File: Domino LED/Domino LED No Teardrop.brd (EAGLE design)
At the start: 27.9 x 10.2 mm, 23 parts, among them J1 MH11-1

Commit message: Changed copyright
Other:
- board text added: "Reference designs are provided "AS IS" and "WITH ALL FAULTS". The Domino Team disclaims all other warranties express or implied, regarding this product, including but not limited to, any implied warranties of merchantibility or fitness for any particular application."
- board text added: "The Domino Team may make changes to specifications and product descriptions at any time, without notice."
- board text added: "© 2014, The Domino Team. All rights reserved."
- board text removed: "Michel Stempin may make changes to specifications and product descriptions at any time, without notice."
- board text removed: "Reference designs are provided "AS IS" and "WITH ALL FAULTS". Michel Stempin disclaims all other warranties express or implied, regarding this product, including but not limited to, any implied warranties of merchantibility or fitness for any particular application."
- board text removed: "© 2014, Michel Stempin. All rights reserved."
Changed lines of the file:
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@@
 See creativecommons.org/licenses/by-sa/4.0/</text>
 <text x="34.29" y="-51.943" size="0.8128" layer="48" ratio="20">Reference designs are provided "AS IS" and "WITH ALL FAULTS".
-Michel Stempin disclaims all other warranties express or implied,
+The Domino Team disclaims all other warranties express or implied,
 regarding this product, including but not limited to, any implied warranties of
 merchantibility or fitness for any particular application.</text>
-<text x="34.29" y="-55.753" size="0.8128" layer="48" ratio="20">Michel Stempin may make changes to specifications and product descriptions
+<text x="34.29" y="-55.753" size="0.8128" layer="48" ratio="20">The Domino Team may make changes to specifications and product descriptions
 at any time, without notice.</text>
-<text x="74.93" y="-41.91" size="1.27" layer="48" ratio="20">© 2014, Michel Stempin.
+<text x="74.93" y="-41.91" size="1.27" layer="48" ratio="20">© 2014, The Domino Team.
 All rights reserved.</text>
 <text x="115.57" y="-57.15" size="1.778" layer="48">Rev.</text>

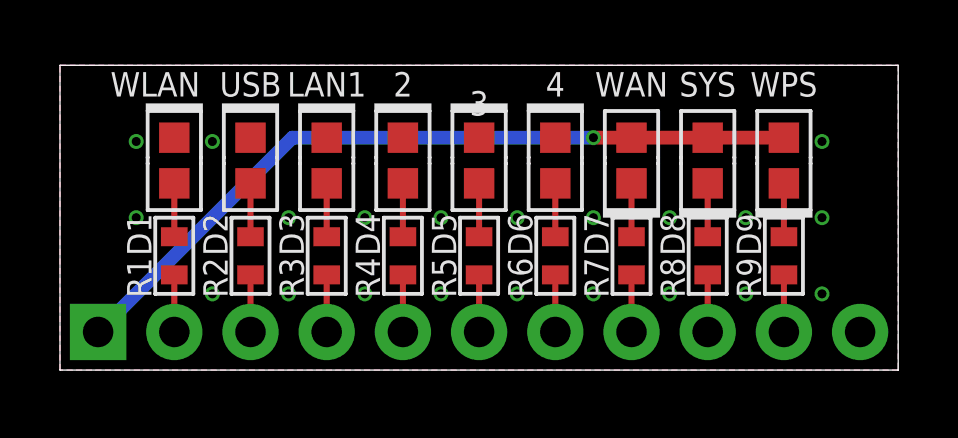
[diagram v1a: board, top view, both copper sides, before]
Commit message: ... and all the files I missed
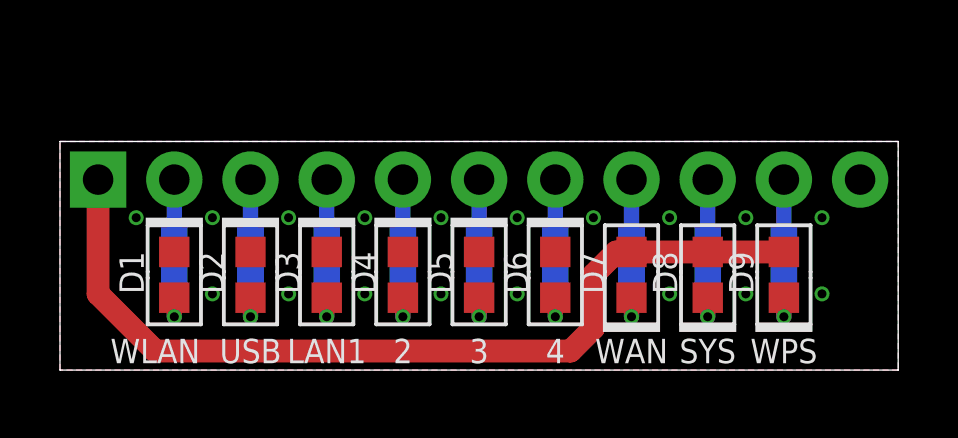
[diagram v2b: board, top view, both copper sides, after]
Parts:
- removed U$4: (no value), Domino:DOMINO_LOGO_SMALL
- moved J1 5.08 mm to (1.27, 6.35)
- moved D1 3.81 mm to (3.81, 3.17)
- moved D2 3.81 mm to (6.35, 3.17)
- moved D3 3.81 mm to (8.89, 3.17)
- moved D4 3.81 mm to (11.4, 3.17)
- moved D5 3.81 mm to (14.0, 3.17)
- moved D6 3.81 mm to (16.5, 3.17)
- moved D7 3.81 mm to (19.1, 3.17)
- moved D8 3.81 mm to (21.6, 3.17)
- moved D9 3.81 mm to (24.1, 3.17)
- moved DRILEGEND 1.27 mm to (81.5, 59.9)
- flipped R1 to the bottom, turned to 270 degrees
- flipped R2 to the bottom, turned to 270 degrees
- flipped R3 to the bottom, turned to 270 degrees
- flipped R4 to the bottom, turned to 270 degrees
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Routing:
- net +3V3: track 25.5 -> 29.9 mm, vias 1 -> 0
- net N$9: track 1.78 -> 2.03 mm, vias 0 -> 1
- net N$8: track 1.78 -> 2.03 mm, vias 0 -> 1
- net N$7: track 1.78 -> 2.03 mm, vias 0 -> 1
- net N$6: track 1.78 -> 2.03 mm, vias 0 -> 1
- net N$5: track 1.78 -> 2.03 mm, vias 0 -> 1
- net N$4: track 1.78 -> 2.03 mm, vias 0 -> 1
- net N$3: track 1.78 -> 2.03 mm, vias 0 -> 1
- net N$2: track 1.78 -> 2.03 mm, vias 0 -> 1
- net N$10: track 1.78 -> 2.03 mm, vias 0 -> 1
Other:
- board size 27.9 x 10.2 mm -> 27.9 x 7.6 mm
- board text removed: "ELD3"
- board text removed: "Rev. A"
